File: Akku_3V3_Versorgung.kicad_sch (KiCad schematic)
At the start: 31 parts, among them J1 Conn_01x03, P1 USB_C_Receptacle_USB2.0_16P, Q1 FS8205A, U1 TP4056, U3 MT3608, U4 AP2112K-3.3, U5 DW01A

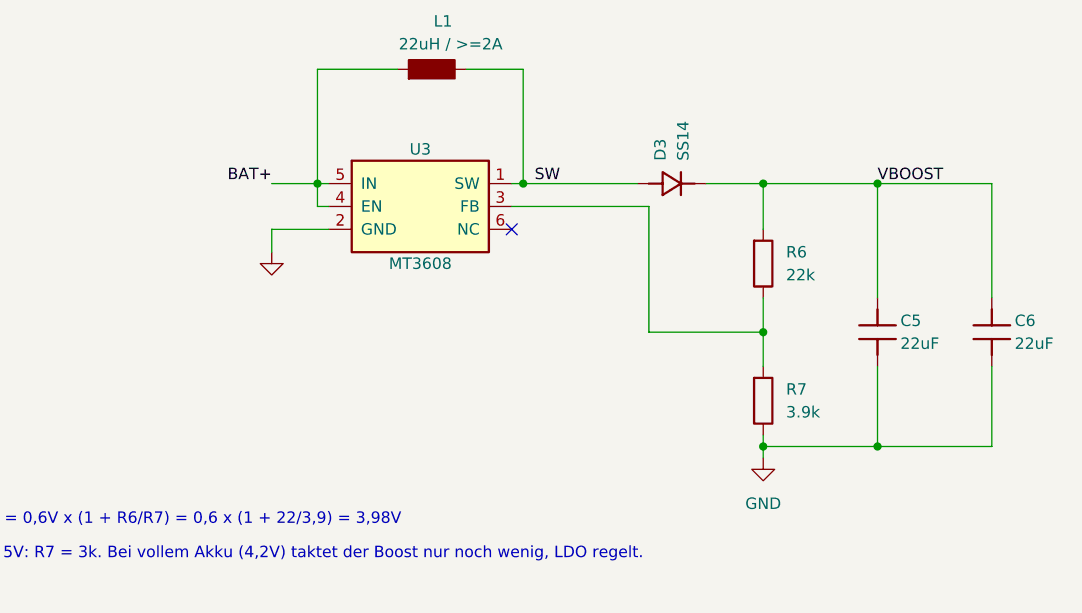
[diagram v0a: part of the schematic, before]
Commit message: shematic review
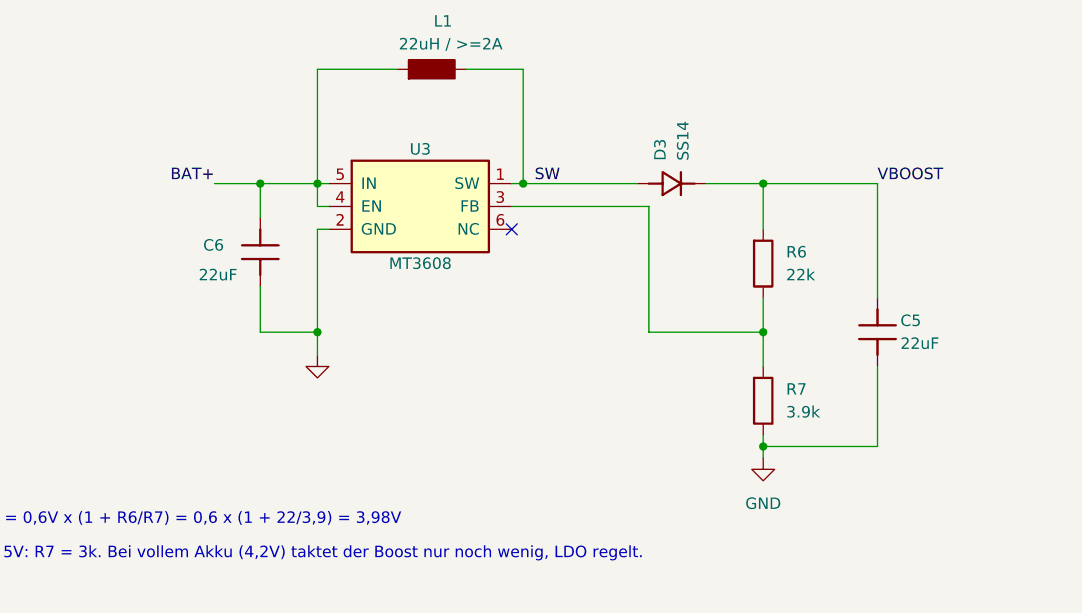
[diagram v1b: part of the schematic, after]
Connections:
- net BAT+: now also C6.1
- net VBOOST: no longer C6.1
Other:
- moved on the sheet: C6
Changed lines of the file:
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@@
 	)
 	(junction
-		(at 274.32 92.71)
+		(at 234.95 63.5)
 		(diameter 0)
 		(color 0 0 0 0)
 	)
 	(junction
-		(at 234.95 63.5)
+		(at 212.09 80.01)
 		(diameter 0)
 		(color 0 0 0 0)
@@
 	)
 	(junction
-		(at 274.32 63.5)
+		(at 261.62 80.01)
 		(diameter 0)
 		(color 0 0 0 0)
 	)
 	(junction
-		(at 261.62 80.01)
+		(at 96.52 172.72)
 		(diameter 0)
 		(color 0 0 0 0)
 	)
 	(junction
-		(at 96.52 172.72)
+		(at 259.08 157.48)
 		(diameter 0)
 		(color 0 0 0 0)
 	)
 	(junction
-		(at 259.08 157.48)
+		(at 205.74 63.5)
 		(diameter 0)
 		(color 0 0 0 0)
@@
 	(wire
 		(pts
+			(xy 205.74 80.01) (xy 212.09 80.01)
+		)
+		(stroke
+			(width 0)
+			(type default)
+		)
+	)
+	(wire
+		(pts
 			(xy 34.29 86.36) (xy 62.23 86.36)
 		)
@@
 	(wire
 		(pts
+			(xy 205.74 63.5) (xy 212.09 63.5)
+		)
+		(stroke
+			(width 0)
+			(type default)
+		)
+	)
+	(wire
+		(pts
 			(xy 46.99 154.94) (xy 46.99 161.29)
 		)
@@
 	(wire
 		(pts
+			(xy 205.74 67.31) (xy 205.74 63.5)
+		)
+		(stroke
+			(width 0)
+			(type default)
+		)
+	)
+	(wire
+		(pts
 			(xy 259.08 172.72) (xy 259.08 173.99)
 		)
@@
 	(wire
 		(pts
-			(xy 207.01 68.58) (xy 207.01 71.12)
-		)
-		(stroke
-			(width 0)
-			(type default)
-		)
-	)
-	(wire
-		(pts
 			(xy 123.19 170.18) (xy 123.19 172.72)
 		)
@@
 	(wire
 		(pts
-			(xy 287.02 92.71) (xy 274.32 92.71)
-		)
-		(stroke
-			(width 0)
-			(type default)
-		)
-	)
-	(wire
-		(pts
 			(xy 46.99 168.91) (xy 46.99 176.53)
 		)
@@
 	(wire
 		(pts
-			(xy 287.02 83.82) (xy 287.02 92.71)
-		)
-		(stroke
-			(width 0)
-			(type default)
-		)
-	)
-	(wire
-		(pts
 			(xy 120.65 167.64) (xy 123.19 167.64)
 		)
@@
 	(wire
 		(pts
-			(xy 107.95 86.36) (xy 82.55 86.36)
+			(xy 205.74 80.01) (xy 205.74 74.93)
 		)
 		(stroke
@@
 	(wire
 		(pts
-			(xy 157.48 69.85) (xy 157.48 78.74)
+			(xy 107.95 86.36) (xy 82.55 86.36)
 		)
 		(stroke
@@
 	(wire
 		(pts
-			(xy 99.06 163.83) (xy 83.82 163.83)
+			(xy 157.48 69.85) (xy 157.48 78.74)
 		)
 		(stroke
@@
 	(wire
 		(pts
-			(xy 194.31 157.48) (xy 194.31 166.37)
+			(xy 99.06 163.83) (xy 83.82 163.83)
 		)
 		(stroke
@@
 	(wire
 		(pts
-			(xy 82.55 66.04) (xy 82.55 86.36)
+			(xy 194.31 157.48) (xy 194.31 166.37)
 		)
 		(stroke
@@
 	(wire
 		(pts
-			(xy 287.02 63.5) (xy 287.02 76.2)
+			(xy 82.55 66.04) (xy 82.55 86.36)
 		)
 		(stroke
@@
 	(wire
 		(pts
-			(xy 207.01 68.58) (xy 213.36 68.58)
+			(xy 212.09 68.58) (xy 213.36 68.58)
 		)
 		(stroke
@@
 	(wire
 		(pts
-			(xy 274.32 63.5) (xy 287.02 63.5)
-		)
-		(stroke
-			(width 0)
-			(type default)
-		)
-	)
-	(wire
-		(pts
 			(xy 213.36 66.04) (xy 212.09 66.04)
 		)
@@
 	(wire
 		(pts
-			(xy 207.01 63.5) (xy 212.09 63.5)
+			(xy 200.66 63.5) (xy 205.74 63.5)
 		)
 		(stroke
@@
 	(wire
 		(pts
+			(xy 212.09 68.58) (xy 212.09 82.55)
+		)
+		(stroke
+			(width 0)
+			(type default)
+		)
+	)
+	(wire
+		(pts
 			(xy 105.41 58.42) (xy 116.84 58.42)
 		)
@@
 	)
 	(label "BAT+"
-		(at 207.01 63.5 180)
+		(at 200.66 63.5 180)
 		(effects
 			(font
@@
 	(symbol
 		(lib_id "Akku3V3:C")
-		(at 287.02 80.01 0)
+		(at 205.74 71.12 0)
 		(unit 1)
 		(body_style 1)
@@
 		(dnp no)
 		(property "Reference" "C6"
-			(at 289.56 78.74 0)
+			(at 199.39 70.358 0)
 			(show_name no)
 			(do_not_autoplace no)
@@
 		)
 		(property "Value" "22uF"
-			(at 289.56 81.28 0)
+			(at 198.882 73.66 0)
 			(show_name no)
 			(do_not_autoplace no)
@@
 		)
 		(property "Footprint" "Capacitor_SMD:C_1206_3216Metric"
-			(at 287.02 80.01 0)
+			(at 205.74 71.12 0)
 			(hide yes)
 			(show_name no)
@@
 		)
 		(property "Datasheet" ""
-			(at 287.02 80.01 0)
+			(at 205.74 71.12 0)
 			(hide yes)
 			(show_name no)
@@
 		)
 		(property "Description" ""
-			(at 287.02 80.01 0)
+			(at 205.74 71.12 0)
 			(hide yes)
 			(show_name no)
@@
 	(symbol
 		(lib_id "power:GND")
-		(at 207.01 71.12 0)
+		(at 212.09 82.55 0)
 		(unit 1)
 		(body_style 1)
@@
 		(fields_autoplaced yes)
 		(property "Reference" "#PWR03"
-			(at 207.01 77.47 0)
+			(at 212.09 88.9 0)
 			(hide yes)
 			(show_name no)
@@
 		)
 		(property "Value" "GND"
-			(at 207.01 76.2 0)
+			(at 212.09 87.63 0)
 			(hide yes)
 			(show_name no)
@@
 		)
 		(property "Footprint" ""
-			(at 207.01 71.12 0)
+			(at 212.09 82.55 0)
 			(hide yes)
 			(show_name no)
@@
 		)
 		(property "Datasheet" ""
-			(at 207.01 71.12 0)
+			(at 212.09 82.55 0)
 			(hide yes)
 			(show_name no)
@@
 		)
 		(property "Description" "Power symbol creates a global label with name \"GND\" , ground"
-			(at 207.01 71.12 0)
+			(at 212.09 82.55 0)
 			(hide yes)
 			(show_name no)

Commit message: shematic review
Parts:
- L1: footprint Inductor_SMD:L_Bourns_SRN6045TA -> Inductor_SMD:L_1206_3216Metric
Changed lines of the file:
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@@
 			)
 		)
-		(property "Footprint" "Inductor_SMD:L_Bourns_SRN6045TA"
+		(property "Footprint" "Inductor_SMD:L_1206_3216Metric"
 			(at 224.79 50.8 0)
 			(hide yes)

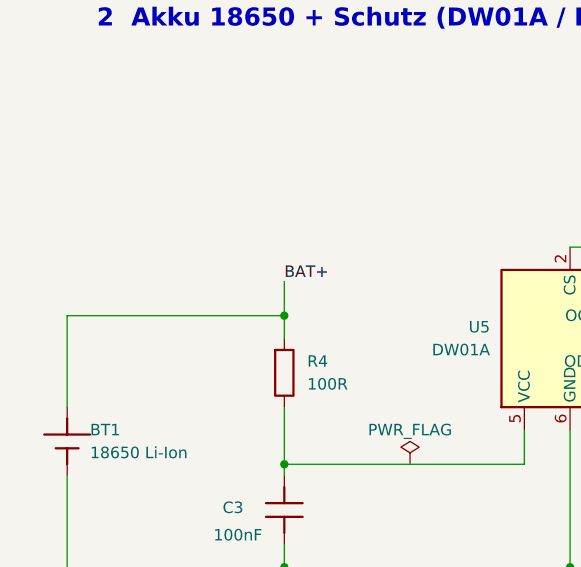
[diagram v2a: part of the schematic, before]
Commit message: shematic review
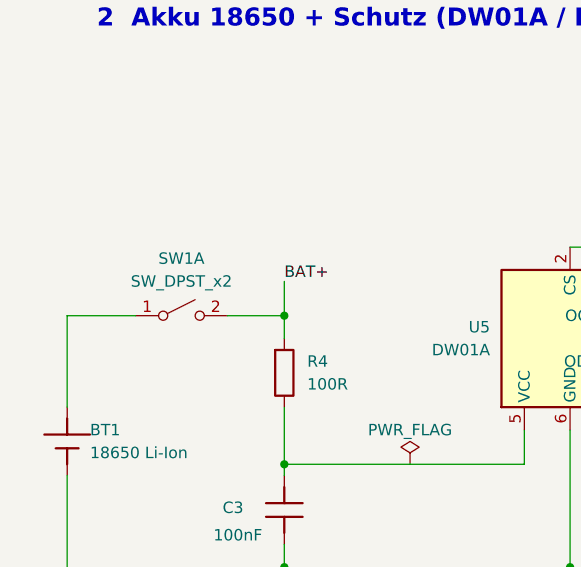
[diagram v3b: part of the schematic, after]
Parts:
- added SW1: SW_DPST_x2, symbol Switch:SW_DPST_x2
- D1, D2: footprint LED_SMD:LED_0603_1608Metric -> LED_THT:LED_D2.0mm_W4.8mm_H2.5mm_FlatTop
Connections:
- net BAT+: now also SW1.2 (B); no longer BT1.1 (+)
- new net: BT1.1 (+), SW1.1 (A)
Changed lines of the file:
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@@
 	(wire
 		(pts
-			(xy 22.86 158.75) (xy 46.99 158.75)
+			(xy 22.86 158.75) (xy 30.48 158.75)
 		)
 		(stroke
@@
 	(wire
 		(pts
+			(xy 40.64 158.75) (xy 46.99 158.75)
+		)
+		(stroke
+			(width 0)
+			(type default)
+		)
+	)
+	(wire
+		(pts
 			(xy 120.65 167.64) (xy 123.19 167.64)
 		)
@@
 			)
 		)
-		(property "Footprint" "LED_SMD:LED_0603_1608Metric"
+		(property "Footprint" "LED_THT:LED_D2.0mm_W4.8mm_H2.5mm_FlatTop"
 			(at 147.32 66.04 0)
 			(hide yes)
@@
 	)
 	(symbol
+		(lib_id "Switch:SW_DPST_x2")
+		(at 35.56 158.75 0)
+		(unit 1)
+		(body_style 1)
+		(exclude_from_sim no)
+		(in_bom yes)
+		(on_board yes)
+		(in_pos_files yes)
+		(dnp no)
+		(fields_autoplaced yes)
+		(property "Reference" "SW1"
+			(at 35.56 152.4 0)
+			(show_name no)
+			(do_not_autoplace no)
+			(effects
+				(font
+					(size 1.27 1.27)
+				)
+			)
+		)
+		(property "Value" "SW_DPST_x2"
+			(at 35.56 154.94 0)
+			(show_name no)
+			(do_not_autoplace no)
+			(effects
+				(font
+					(size 1.27 1.27)
+				)
+			)
+		)
+		(property "Footprint" ""
+			(at 35.56 158.75 0)
+			(hide yes)
+			(show_name no)
+			(do_not_autoplace no)
+			(effects
+				(font
+					(size 1.27 1.27)
+				)
+			)
+		)
+		(property "Datasheet" ""
+			(at 35.56 158.75 0)
+			(hide yes)
+			(show_name no)
+			(do_not_autoplace no)
+			(effects
+				(font
+					(size 1.27 1.27)
+				)
+			)
+		)
+		(property "Description" "Single Pole Single Throw (SPST) switch, separate symbol"
+			(at 35.56 158.75 0)
+			(hide yes)
+			(show_name no)
+			(do_not_autoplace no)
+			(effects
+				(font
+					(size 1.27 1.27)
+				)
+			)
+		)
+		(pin "1"
+		)
+		(pin "3"
+		)
+		(pin "2"
+		)
+		(pin "4"
+		)
+		(instances
+			(project "Akku_3V3_Versorgung"
+				(path "/75321e38-43b6-49a3-b59a-8489ddbdc7b9"
+					(reference "SW1")
+					(unit 1)
+				)
+			)
+		)
+	)
+	(symbol
 		(lib_id "Akku3V3:C")
 		(at 274.32 80.01 0)
@@
 			)
 		)
-		(property "Footprint" "LED_SMD:LED_0603_1608Metric"
+		(property "Footprint" "LED_THT:LED_D2.0mm_W4.8mm_H2.5mm_FlatTop"
 			(at 157.48 66.04 0)
 			(hide yes)

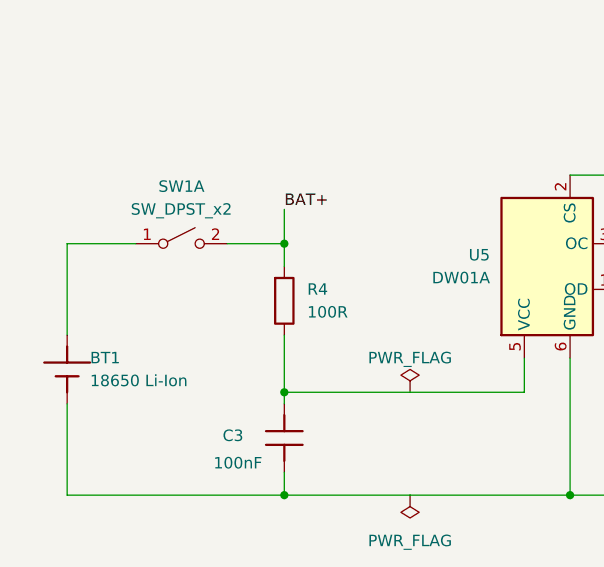
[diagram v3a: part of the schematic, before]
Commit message: shematic review
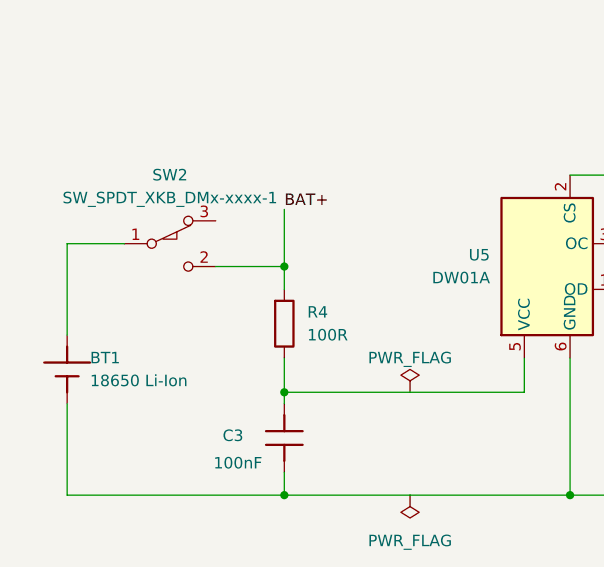
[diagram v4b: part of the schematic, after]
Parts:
- removed SW1: SW_DPST_x2, symbol Switch:SW_DPST_x2
- added SW2: SW_SPDT_XKB_DMx-xxxx-1, PCM_yvolodym:Switch_Small, symbol Switch:SW_SPDT_XKB_DMx-xxxx-1
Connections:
- net BAT+: now also SW2.2 (B)
- net at BT1.1 (+): now also SW2.1 (A)
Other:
- moved on the sheet: R4
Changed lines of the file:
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@@
 	)
 	(junction
-		(at 46.99 158.75)
+		(at 46.99 161.29)
 		(diameter 0)
 		(color 0 0 0 0)
@@
 	(wire
 		(pts
-			(xy 22.86 158.75) (xy 30.48 158.75)
-		)
-		(stroke
-			(width 0)
-			(type default)
-		)
-	)
-	(wire
-		(pts
 			(xy 129.54 151.13) (xy 129.54 154.94)
 		)
@@
 	(wire
 		(pts
-			(xy 46.99 168.91) (xy 46.99 176.53)
+			(xy 46.99 171.45) (xy 46.99 176.53)
 		)
 		(stroke
@@
 	(wire
 		(pts
-			(xy 40.64 158.75) (xy 46.99 158.75)
+			(xy 120.65 167.64) (xy 123.19 167.64)
 		)
 		(stroke
@@
 	(wire
 		(pts
-			(xy 120.65 167.64) (xy 123.19 167.64)
+			(xy 67.31 60.96) (xy 67.31 86.36)
 		)
 		(stroke
@@
 	(wire
 		(pts
-			(xy 67.31 60.96) (xy 67.31 86.36)
+			(xy 72.39 63.5) (xy 85.09 63.5)
 		)
 		(stroke
@@
 	(wire
 		(pts
-			(xy 72.39 63.5) (xy 85.09 63.5)
+			(xy 120.65 177.8) (xy 123.19 177.8)
 		)
 		(stroke
@@
 	(wire
 		(pts
-			(xy 120.65 177.8) (xy 123.19 177.8)
+			(xy 39.37 161.29) (xy 46.99 161.29)
 		)
 		(stroke
@@
 	(wire
 		(pts
+			(xy 46.99 161.29) (xy 46.99 163.83)
+		)
+		(stroke
+			(width 0)
+			(type default)
+		)
+	)
+	(wire
+		(pts
 			(xy 212.09 68.58) (xy 213.36 68.58)
 		)
@@
 	(wire
 		(pts
+			(xy 22.86 158.75) (xy 29.21 158.75)
+		)
+		(stroke
+			(width 0)
+			(type default)
+		)
+	)
+	(wire
+		(pts
 			(xy 22.86 158.75) (xy 22.86 168.91)
 		)
@@
 	)
 	(symbol
-		(lib_id "Switch:SW_DPST_x2")
-		(at 35.56 158.75 0)
-		(unit 1)
-		(body_style 1)
-		(exclude_from_sim no)
-		(in_bom yes)
-		(on_board yes)
-		(in_pos_files yes)
-		(dnp no)
-		(fields_autoplaced yes)
-		(property "Reference" "SW1"
-			(at 35.56 152.4 0)
-			(show_name no)
-			(do_not_autoplace no)
-			(effects
-				(font
-					(size 1.27 1.27)
-				)
-			)
-		)
-		(property "Value" "SW_DPST_x2"
-			(at 35.56 154.94 0)
-			(show_name no)
-			(do_not_autoplace no)
-			(effects
-				(font
-					(size 1.27 1.27)
-				)
-			)
-		)
-		(property "Footprint" ""
-			(at 35.56 158.75 0)
-			(hide yes)
-			(show_name no)
-			(do_not_autoplace no)
-			(effects
-				(font
-					(size 1.27 1.27)
-				)
-			)
-		)
-		(property "Datasheet" ""
-			(at 35.56 158.75 0)
-			(hide yes)
-			(show_name no)
-			(do_not_autoplace no)
-			(effects
-				(font
-					(size 1.27 1.27)
-				)
-			)
-		)
-		(property "Description" "Single Pole Single Throw (SPST) switch, separate symbol"
-			(at 35.56 158.75 0)
-			(hide yes)
-			(show_name no)
-			(do_not_autoplace no)
-			(effects
-				(font
-					(size 1.27 1.27)
-				)
-			)
-		)
-		(pin "1"
-		)
-		(pin "3"
-		)
-		(pin "2"
-		)
-		(pin "4"
-		)
-		(instances
-			(project "Akku_3V3_Versorgung"
-				(path "/75321e38-43b6-49a3-b59a-8489ddbdc7b9"
-					(reference "SW1")
-					(unit 1)
-				)
-			)
-		)
-	)
-	(symbol
 		(lib_id "Akku3V3:C")
 		(at 274.32 80.01 0)
@@
 	(symbol
 		(lib_id "Akku3V3:R")
-		(at 46.99 165.1 0)
+		(at 46.99 167.64 0)
 		(unit 1)
 		(body_style 1)
@@
 		(dnp no)
 		(property "Reference" "R4"
-			(at 49.53 163.83 0)
+			(at 49.53 166.37 0)
 			(show_name no)
 			(do_not_autoplace no)
@@
 		)
 		(property "Value" "100R"
-			(at 49.53 166.37 0)
+			(at 49.53 168.91 0)
 			(show_name no)
 			(do_not_autoplace no)
@@
 		)
 		(property "Footprint" "Resistor_SMD:R_1206_3216Metric"
-			(at 46.99 165.1 0)
+			(at 46.99 167.64 0)
 			(hide yes)
 			(show_name no)
@@
 		)
 		(property "Datasheet" ""
-			(at 46.99 165.1 0)
+			(at 46.99 167.64 0)
 			(hide yes)
 			(show_name no)
@@
 		)
 		(property "Description" ""
-			(at 46.99 165.1 0)
+			(at 46.99 167.64 0)
 			(hide yes)
 			(show_name no)
@@
 					(unit 1)
 				)
+			)
+		)
+	)
+	(symbol
+		(lib_id "Switch:SW_SPDT_XKB_DMx-xxxx-1")
+		(at 34.29 158.75 0)
+		(unit 1)
+		(body_style 1)
+		(exclude_from_sim no)
+		(in_bom yes)
+		(on_board yes)
+		(in_pos_files yes)
+		(dnp no)
+		(fields_autoplaced yes)
+		(property "Reference" "SW2"
+			(at 34.29 151.13 0)
+			(show_name no)
+			(do_not_autoplace no)
+			(effects
+				(font
+					(size 1.27 1.27)
+				)
+			)
+		)
+		(property "Value" "SW_SPDT_XKB_DMx-xxxx-1"
+			(at 34.29 153.67 0)
+			(show_name no)
+			(do_not_autoplace no)
+			(effects
+				(font
+					(size 1.27 1.27)
+				)
+			)
+		)
+		(property "Footprint" "PCM_yvolodym:Switch_Small"
+			(at 34.29 158.75 0)
+			(hide yes)
+			(show_name no)
+			(do_not_autoplace no)
+			(effects
+				(font
+					(size 1.27 1.27)
+				)
+			)
+		)
+		(property "Datasheet" ""
+			(at 34.29 158.75 0)
+			(hide yes)
+			(show_name no)
+			(do_not_autoplace no)
+			(effects
+				(font
+					(size 1.27 1.27)
+				)
+			)
+		)
+		(property "Description" "Position switch"
+			(at 34.29 158.75 0)
+			(hide yes)
+			(show_name no)
+			(do_not_autoplace no)
+			(effects
+				(font
+					(size 1.27 1.27)
+				)
+			)
+		)
+		(pin "1"
+		)
+		(pin "2"
+		)
+		(pin "3"
+		)
+		(instances
+			(project "Akku_3V3_Versorgung"
+				(path "/75321e38-43b6-49a3-b59a-8489ddbdc7b9"
+					(reference "SW2")
+					(unit 1)
+				)
